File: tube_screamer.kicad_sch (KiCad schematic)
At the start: 40 parts, among them Q1 BC817, U1 TL072

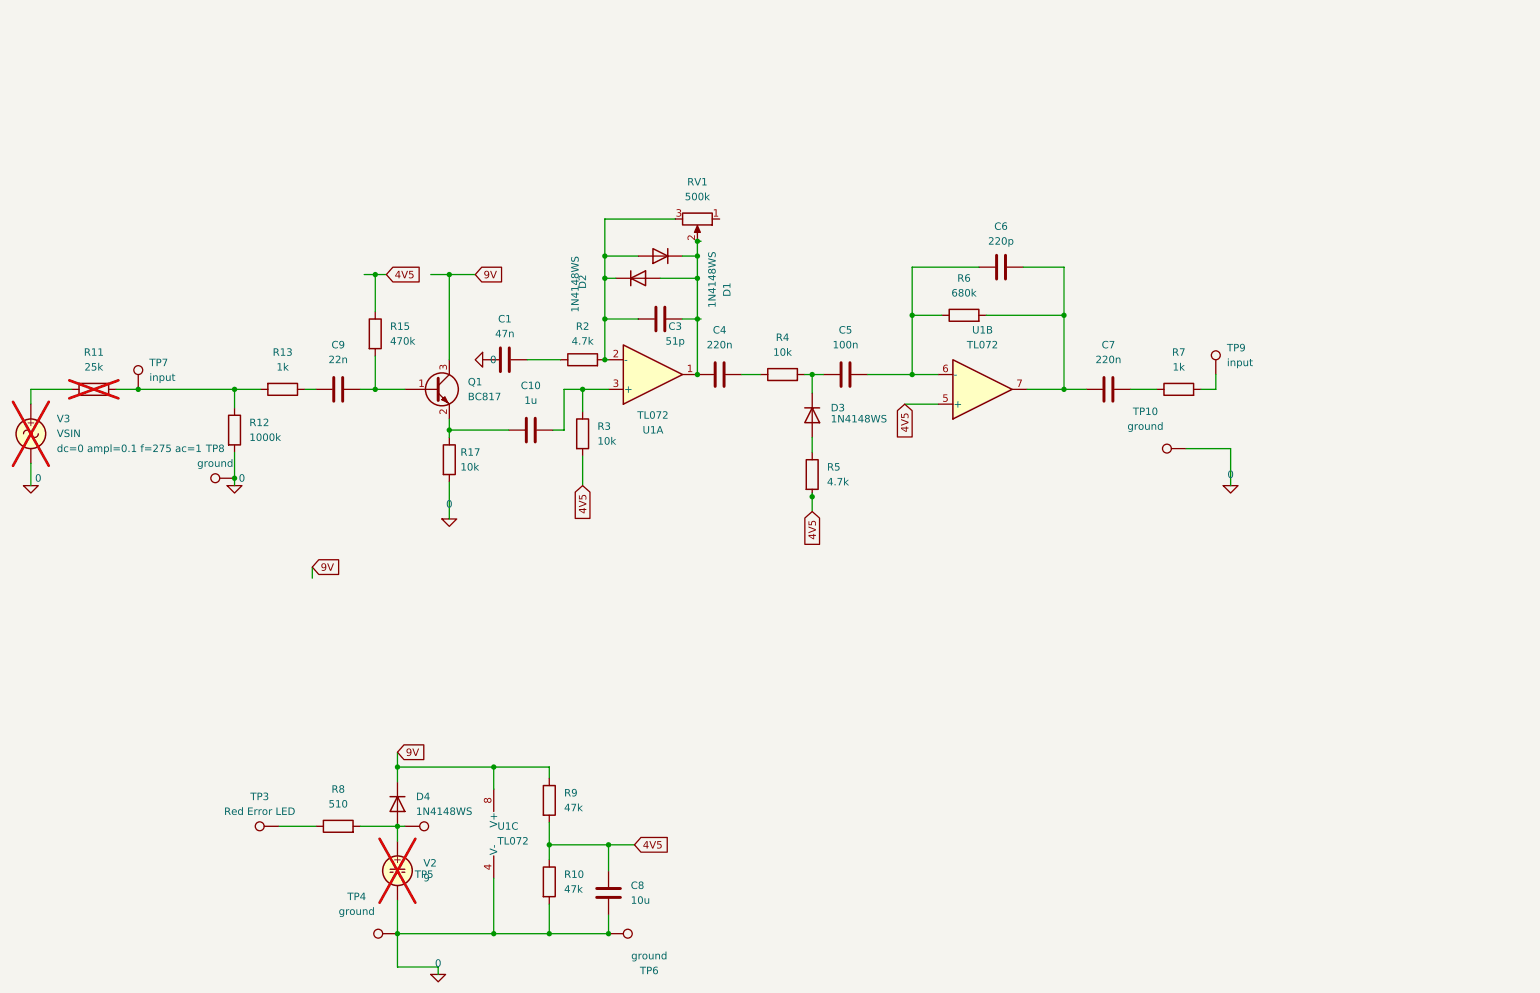
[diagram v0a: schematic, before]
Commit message: Updated schematic
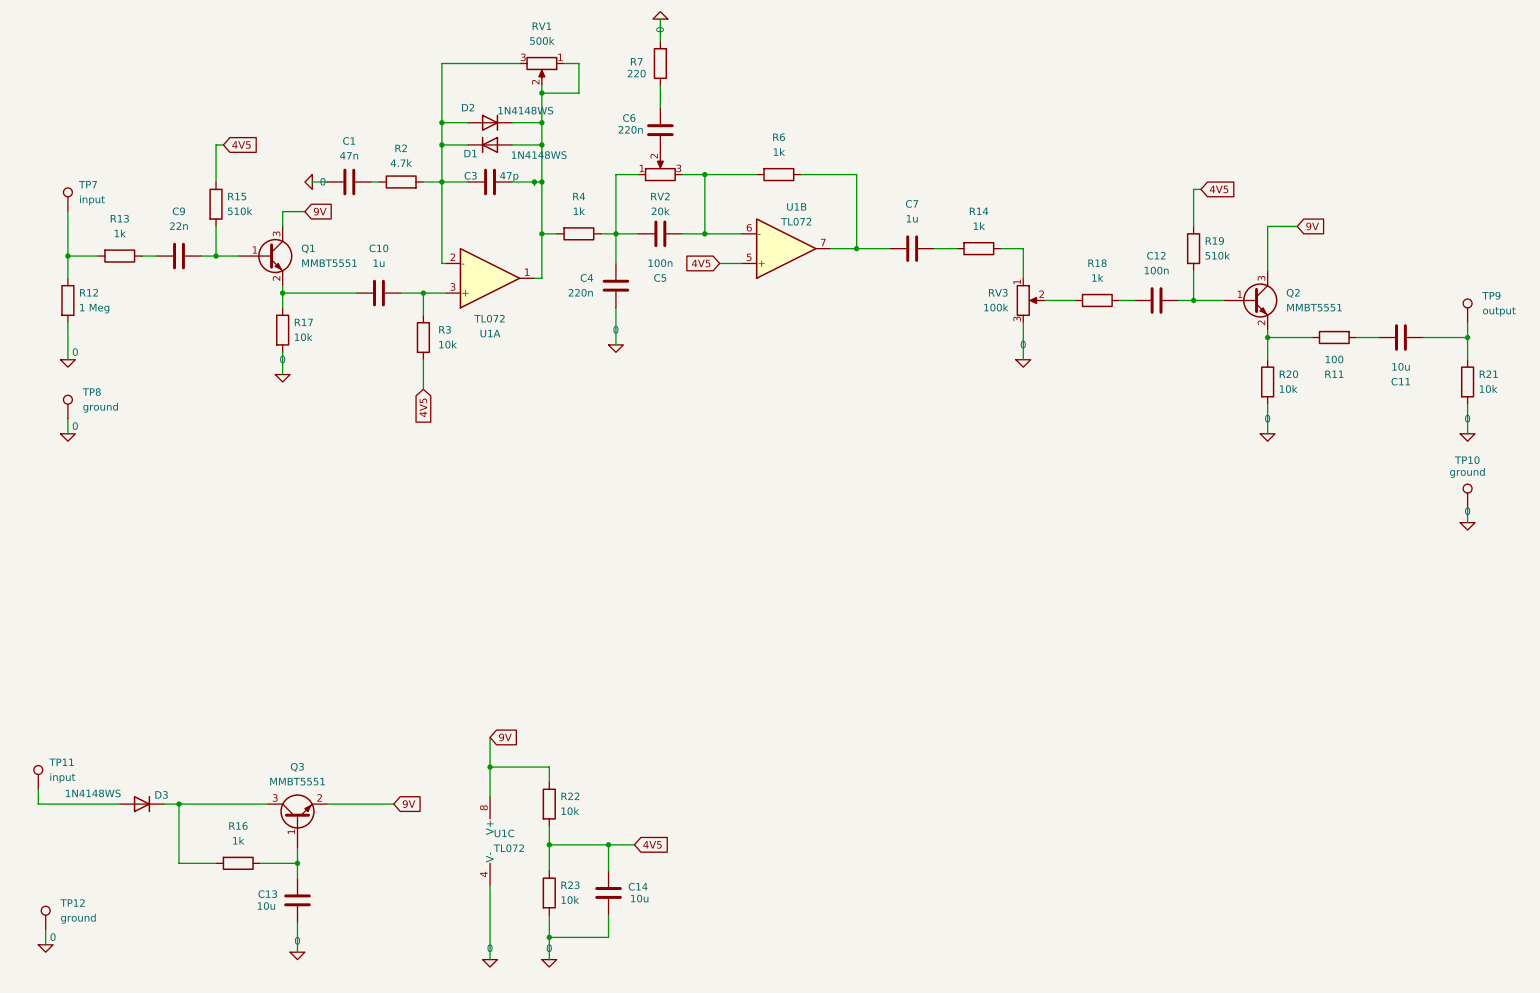
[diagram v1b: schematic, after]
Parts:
- removed C8: 10u, Capacitor_SMD:C_0603_1608Metric_Pad1.08x0.95mm_HandSolder, symbol Device:C
- removed D4: 1N4148WS, Diode_SMD:D_SOD-323, symbol Diode:1N4148WS
- removed R10, R9: 47k, Resistor_SMD:R_0603_1608Metric_Pad0.98x0.95mm_HandSolder, symbol Device:R
- removed R5: 4.7k, Resistor_SMD:R_0603_1608Metric_Pad0.98x0.95mm_HandSolder, symbol Device:R
- removed R8: 510, Resistor_SMD:R_0603_1608Metric_Pad0.98x0.95mm_HandSolder, symbol Device:R
- removed TP3: Red Error LED, TestPoint:TestPoint_Pad_2.0x2.0mm, symbol Connector:TestPoint
- removed TP4, TP6: ground, TestPoint:TestPoint_Pad_2.0x2.0mm, symbol Connector:TestPoint
- removed TP5: Power Supply, TestPoint:TestPoint_Pad_2.0x2.0mm, symbol Connector:TestPoint
- removed V2: 9, symbol Simulation_SPICE:VDC
- removed V3: VSIN, symbol Simulation_SPICE:VSIN
- added C11, C13, C14: 10u, Capacitor_SMD:C_0603_1608Metric_Pad1.08x0.95mm_HandSolder, symbol Device:C
- added C12: 100n, Capacitor_SMD:C_0603_1608Metric_Pad1.08x0.95mm_HandSolder, symbol Device:C
- added Q2, Q3: MMBT5551, Package_TO_SOT_SMD:SOT-23, symbol Transistor_BJT:BC817
- added R14, R16, R18: 1k, Resistor_SMD:R_0603_1608Metric_Pad0.98x0.95mm_HandSolder, symbol Device:R
- added R19: 510k, Resistor_SMD:R_0603_1608Metric_Pad0.98x0.95mm_HandSolder, symbol Device:R
- added R20, R21, R22, R23: 10k, Resistor_SMD:R_0603_1608Metric_Pad0.98x0.95mm_HandSolder, symbol Device:R
- added RV2: 20k, Potentiometer_THT:Potentiometer_Alpha_RD901F-40-00D_Single_Vertical, symbol Device:R_Potentiometer
- added RV3: 100k, Potentiometer_THT:Potentiometer_Alpha_RD901F-40-00D_Single_Vertical, symbol Device:R_Potentiometer
- added TP11: input, TestPoint:TestPoint_Pad_2.0x2.0mm, symbol Connector:TestPoint
- added TP12: ground, TestPoint:TestPoint_Pad_2.0x2.0mm, symbol Connector:TestPoint
- C1: LCSC (none) -> C1622
- C10: LCSC (none) -> C15849
- C3: value 51p -> 47p; LCSC (none) -> C1671
- C4: LCSC (none) -> C21120
- C5: LCSC (none) -> C14663
- C6: value 220p -> 220n; LCSC (none) -> C21120
- C7: value 220n -> 1u; LCSC (none) -> C15849
- C9: LCSC (none) -> C21122
- D1, D2, D3: LCSC (none) -> C2128
- Q1: value BC817 -> MMBT5551; LCSC (none) -> C2145
- R11: value 25k -> 100; footprint Resistor_SMD:R_0402_1005Metric -> Resistor_SMD:R_0603_1608Metric_Pad0.98x0.95mm_HandSolder; LCSC (none) -> C22775; now fitted; now in the parts list
- R12: value 1000k -> 1 Meg; LCSC (none) -> C22935
- R13: LCSC (none) -> C21190
- R15: value 470k -> 510k; LCSC (none) -> C23192
- R17, R3: LCSC (none) -> C25804
- R2: LCSC (none) -> C23162
- R4: value 10k -> 1k; LCSC (none) -> C21190
- R6: value 680k -> 1k; LCSC (none) -> C21190
- R7: value 1k -> 220; LCSC (none) -> C25804
- TP9: value input -> output
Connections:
- net 0: now also C4.1, R7.2, C13.2, C14.2, R20.2, R21.2, R23.2, RV3.3, TP12.1
- net 4V5: now also C14.1, R19.1, R22.2, R23.1
- net 9V: now also Q2.3 (C), Q3.2 (E), R22.1
- net at C3.2, D1.2 (A), D2.1 (K)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: now also R4.2, RV1.1; no longer C4.1
- net at C7.2: now also R14.2; no longer R7.1
- net at TP9.1: now also C11.2, R21.1; no longer R7.2
- net at C5.2, U1.6 (-): now also R6.2, RV2.3; no longer C6.1, R6.1
- net at C7.1, U1.7: now also R6.1; no longer C6.2, R6.2
- net at D3.2 (A): now also TP11.1
- net at C4.2, R4.1: now also C5.1, RV2.1
- net at R11.2: now also C11.1
- net at R12.1, R13.2, TP7.1: no longer R11.1
- new net: C13.1, Q3.1 (B), R16.1
- new net: D3.1 (K), Q3.3 (C), R16.2
- new net: C12.2, Q2.1 (B), R19.2
- new net: Q2.2 (E), R11.1, R20.1
- new net: R14.1, RV3.1
- new net: R18.2, RV3.2
- new net: C12.1, R18.1
- new net: C6.1, RV2.2
- new net: C6.2, R7.1
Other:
- moved on the sheet: C1, C10, C3, C5, C9, D1, Q1, R12, R13, R15, R17, R2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
